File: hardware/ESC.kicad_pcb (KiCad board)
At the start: 4 copper layers, 52 x 25 mm, 89 parts, among them J1 +, J10 +, J2 -, J3 +, J4 +, J5 +, J6 +, J7 Conn_01x03, J8 +, J9 +, Q1 AGM60P30AP, Q2 AGM60P30AP, Q3 AGM60P30AP, Q4 AGM60P30AP, Q5 AGM60P30AP, Q6 AGM60P30AP, Q7 AGM60P30A, SW3 SW_Push, U1 DRV8323RSRGZR, U2 STM32G431CBTx, Y1 X322516MLB4SI

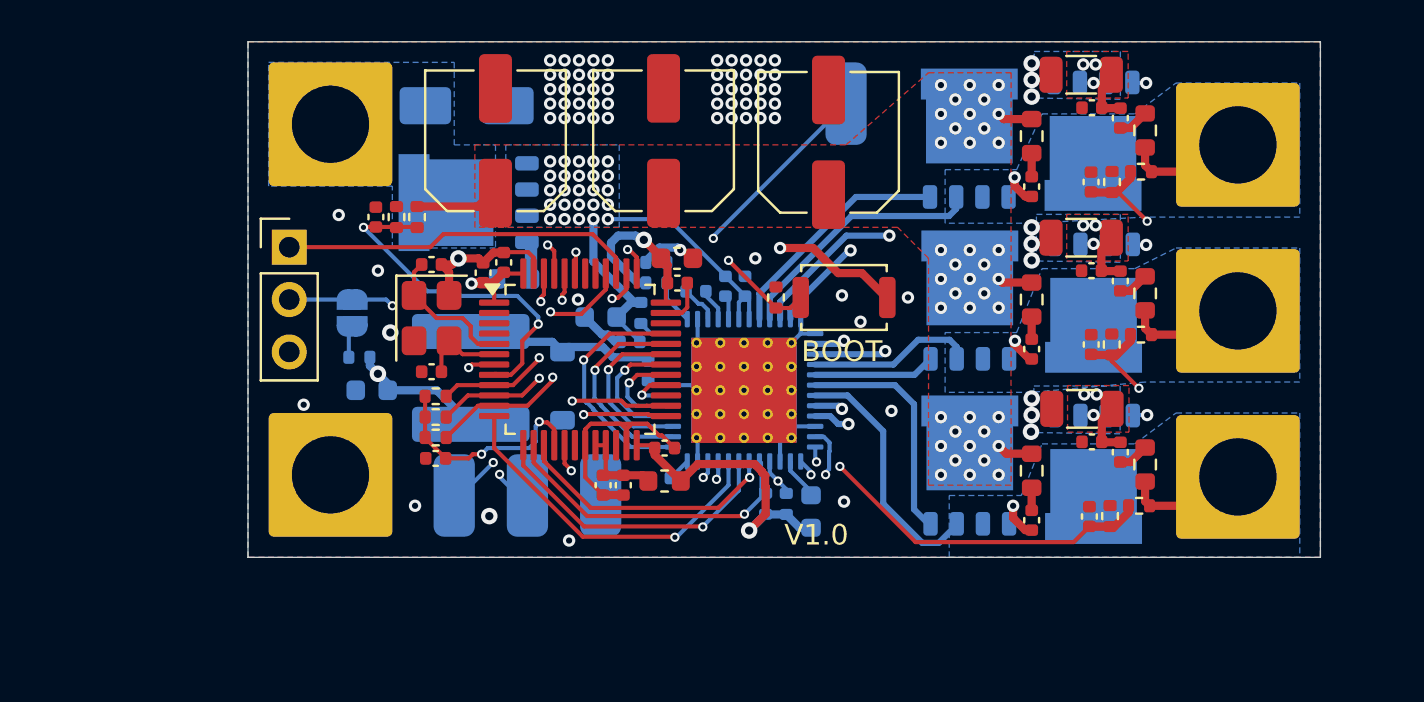
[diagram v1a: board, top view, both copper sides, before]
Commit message: made pcb layout
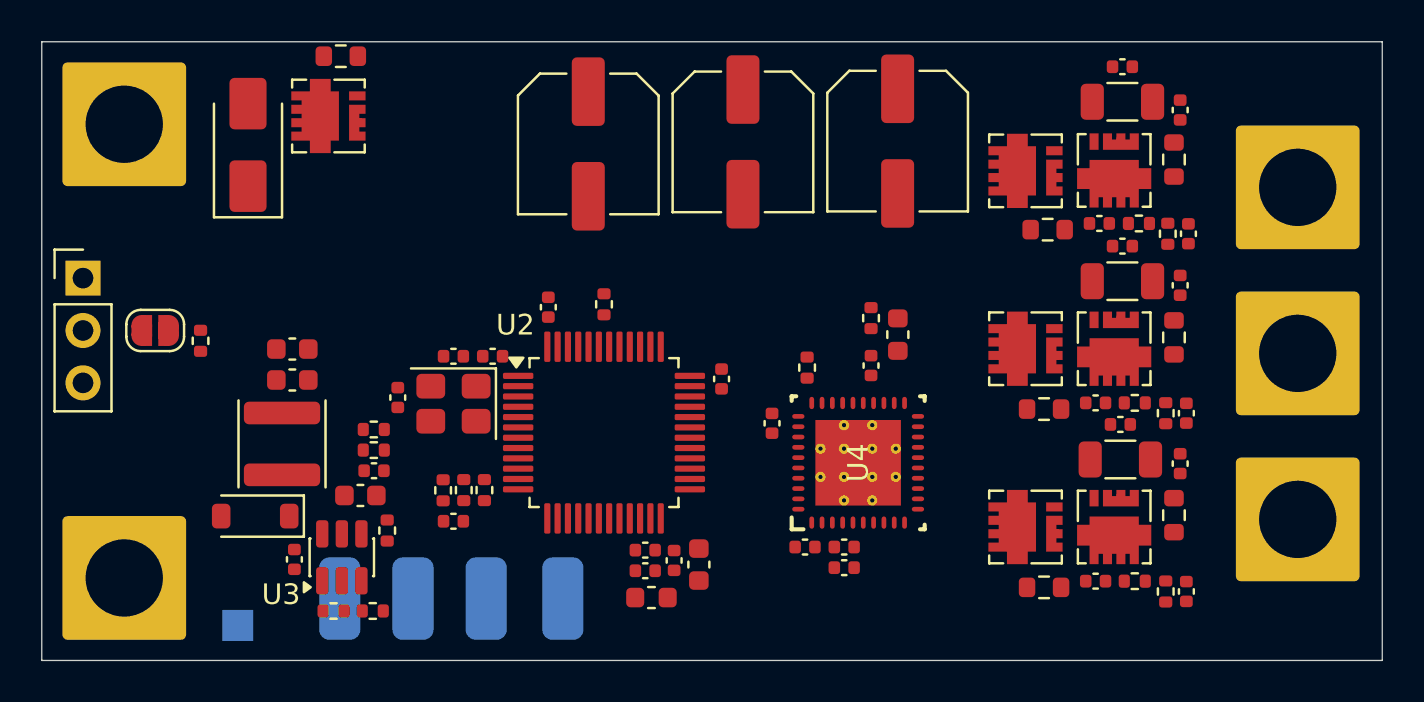
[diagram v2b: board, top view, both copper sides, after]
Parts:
- removed C10, C7: 100nF, Capacitor_SMD:C_0402_1005Metric
- removed C12, C13: 1uF, Capacitor_SMD:C_0402_1005Metric
- removed C14: 2.2uF, Capacitor_SMD:C_0603_1608Metric
- removed C8: 10uF, Capacitor_SMD:C_0603_1608Metric
- removed R10: 100K, Resistor_SMD:R_0402_1005Metric
- removed R11: 3.3K, Resistor_SMD:R_0402_1005Metric
- removed R12: 1K, Resistor_SMD:R_0402_1005Metric
- removed R14, R15: 10k, Resistor_SMD:R_0402_1005Metric
- removed SW3: SW_Push, Button_Switch_SMD:SW_Push_SPST_NO_Alps_SKRK
- removed U1: DRV8323RSRGZR, Package_DFN_QFN:QFN-48-1EP_7x7mm_P0.5mm_EP5.1x5.1mm_ThermalVias
- added C37: 10uF, Capacitor_SMD:C_0603_1608Metric, F.Cu at (143.4, 107.0)
- added C38: 15uF, Capacitor_SMD:C_0603_1608Metric, F.Cu at (140.2, 101.4)
- added C39: 15uF, Capacitor_SMD:C_0603_1608Metric, F.Cu at (140.2, 99.9)
- added C40: 100nF, Capacitor_SMD:C_0402_1005Metric, F.Cu at (140.2, 110.1)
- added C41: 100nF, Capacitor_SMD:C_0402_1005Metric, F.Cu at (168.2, 100.7)
- added C42: 1uF, Capacitor_SMD:C_0402_1005Metric, F.Cu at (163.4, 103.5)
- added C43: 100nF, Capacitor_SMD:C_0402_1005Metric, F.Cu at (166.9, 110.5)
- added R29: 28K, Resistor_SMD:R_0402_1005Metric, F.Cu at (142.2, 112.6)
- added R30: 8.45K, Resistor_SMD:R_0402_1005Metric, F.Cu at (144.1, 112.6)
- added R31: 10k, Resistor_SMD:R_0402_1005Metric, F.Cu at (168.2, 98.4)
- added R32: 100K, Resistor_SMD:R_0402_1005Metric, F.Cu at (165.1, 100.8)
- added R33: 10k, Resistor_SMD:R_0402_1005Metric, F.Cu at (155.3, 97.7)
- added TP1: TestPoint, TestPoint:TestPoint_Pad_1.5x1.5mm, B.Cu at (137.5, 113.3)
- added U3: LMR16006X, Package_TO_SOT_SMD:SOT-23-6, F.Cu at (142.6, 110.0)
- added U4: DRV8323SRTAR, ESC-footprints:DRV8323SRTAR, F.Cu at (167.6, 105.4)
- C11, D1, D2, FB1, JP1, R13, R20: moved to F.Cu
- C9: value 100nF -> 1uF; moved to F.Cu
- L1: value 22uH -> 27uH; footprint Inductor_SMD:L_APV_ANR6020 -> Inductor_SMD:L_APV_ANR4030; moved to F.Cu
- Q1, Q2, Q3, Q4, Q5, Q6: value AGM60P30AP -> AGM60P30A; footprint Package_DFN_QFN:PQFN-8-EP_6x5mm_P1.27mm_Generic -> Diode_SMD:D_QFN_3.3x3.3mm_P0.65mm; moved to F.Cu
- Q7: footprint Package_DFN_QFN:PQFN-8-EP_6x5mm_P1.27mm_Generic -> Diode_SMD:D_QFN_3.3x3.3mm_P0.65mm; moved to F.Cu
- R16, R18, R21, R22, R24, R26, R27: value 162K -> 226K
- R17, R19, R23, R25: value 20K -> 28K
- R28: value 10K -> 100K
- moved J10 27.7 mm to (153.3, 112.0)
- moved R28 22.0 mm to (144.8, 108.7), turned to -90 degrees
- moved C20 19.5 mm to (169.5, 89.8), turned to -90 degrees
- moved Q1 18.9 mm to (175.7, 108.5), turned to 0 degrees
- moved D1 16.2 mm to (138.3, 108.0), turned to 180 degrees
- moved C29 14.9 mm to (159.9, 110.3), turned to -90 degrees
- moved Q5 14.6 mm to (175.7, 91.3), turned to 0 degrees
- moved C9 14.4 mm to (166.9, 109.5)
- moved R13 13.7 mm to (142.5, 85.7)
- moved J9 13.6 mm to (142.4, 112.0), turned to 180 degrees
- moved C11 13.5 mm to (165.0, 109.5)
- moved C26 13.5 mm to (158.7, 110.2), turned to -90 degrees
- moved C32 12.3 mm to (144.1, 105.8), turned to 180 degrees
- moved C18 11.7 mm to (154.5, 90.0), turned to -90 degrees
- moved R25 11.4 mm to (144.1, 104.8), turned to 180 degrees
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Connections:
- net /BGND renamed Net-(D1-K)
- C9 pad 2: GND -> Net-(U4-VCP)
- R28 pad 1: /BOOT -> VBUS
- R28 pad 2: GND -> Net-(U3-~{SHDN})
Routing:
- net +3.3V: track 52.3 -> 0.00 mm, vias 6 -> 0
- net GND: track 48.8 -> 0.00 mm, vias 74 -> 0
- net /BEMF_A: track 42.7 -> 0.00 mm, vias 2 -> 0
- net /BEMF_B: track 41.5 -> 0.00 mm, vias 2 -> 0
- net /BEMF_C: track 38.6 -> 0.00 mm, vias 2 -> 0
- net VBUS: track 29.3 -> 0.00 mm, vias 64 -> 0
- net /RESET: track 26.6 -> 0.00 mm, vias 2 -> 0
- net /MOTOR_A: track 26.1 -> 0.00 mm, vias 1 -> 0
- net /DRV_EN: track 25.7 -> 0.00 mm, vias 2 -> 0
- net /GLA: track 23.9 -> 0.00 mm, vias 2 -> 0
- net /DRV_CAL: track 23.8 -> 0.00 mm, vias 2 -> 0
- net /FAULT: track 23.7 -> 0.00 mm, vias 2 -> 0
- net /SPA: track 22.5 -> 0.00 mm, vias 4 -> 0
- net /GLC: track 21.0 -> 0.00 mm, vias 2 -> 0
- net /MOTOR_C: track 20.2 -> 0.00 mm, vias 1 -> 0
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- removed copper zone on In2.Cu, net +3.3V
- removed copper zone on B.Cu, net /MOTOR_A
- removed copper zone on B.Cu, net /MOTOR_B
- removed copper zone on B.Cu, net /MOTOR_C
- removed copper zone on B.Cu, net /SPA
- removed copper zone on F.Cu, net /SPA
- removed copper zone on B.Cu, net /SPB
- removed copper zone on F.Cu, net /SPB
- removed copper zone on B.Cu, net /SPC
- removed copper zone on F.Cu, net /SPC
- removed copper zone on B.Cu, net GND
- removed copper zone on F.Cu, net GND
- removed copper zone on In1.Cu, net GND
- removed copper zone on B.Cu, net Net-(D2-A2)
- removed copper zone on B.Cu, net VBUS
- removed copper zone on F.Cu, net VBUS
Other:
- board size 52 x 25 mm -> 65 x 30 mm
- board text removed: "BOOT"
- board text removed: "CCW"
- board text removed: "CW"
- board text removed: "GND"
- board text removed: "RST"
- board text removed: "SWCLK"
- board text removed: "SWDIO"
- board text removed: "V1.0"
